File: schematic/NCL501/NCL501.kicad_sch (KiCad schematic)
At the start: 24 parts, among them CN1 SCSI Intern, J1 SCSI extern, J2 Bus_ISA_8bit, U1 74LS175, U10 PAL16L8, U2 74LS125, U3 74LS14, U4 6116, U5 53C80, U6 27C128, U7 74LS688, U8 74LS688, U9 74LS245

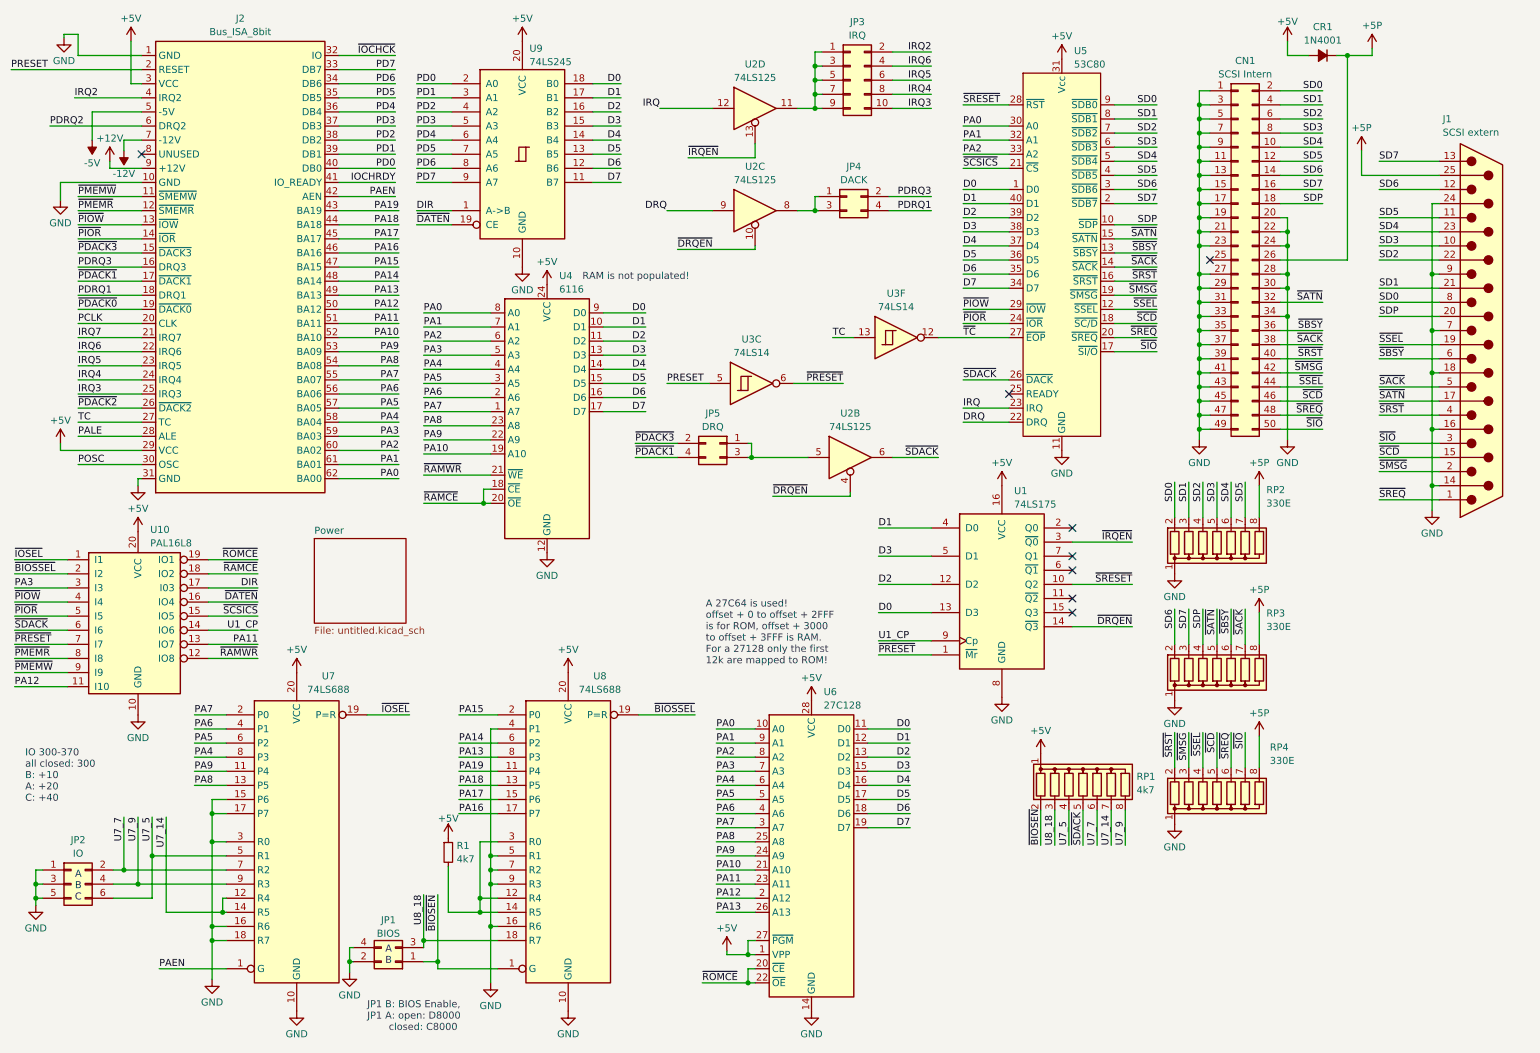
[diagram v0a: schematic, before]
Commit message: first manufactured Version
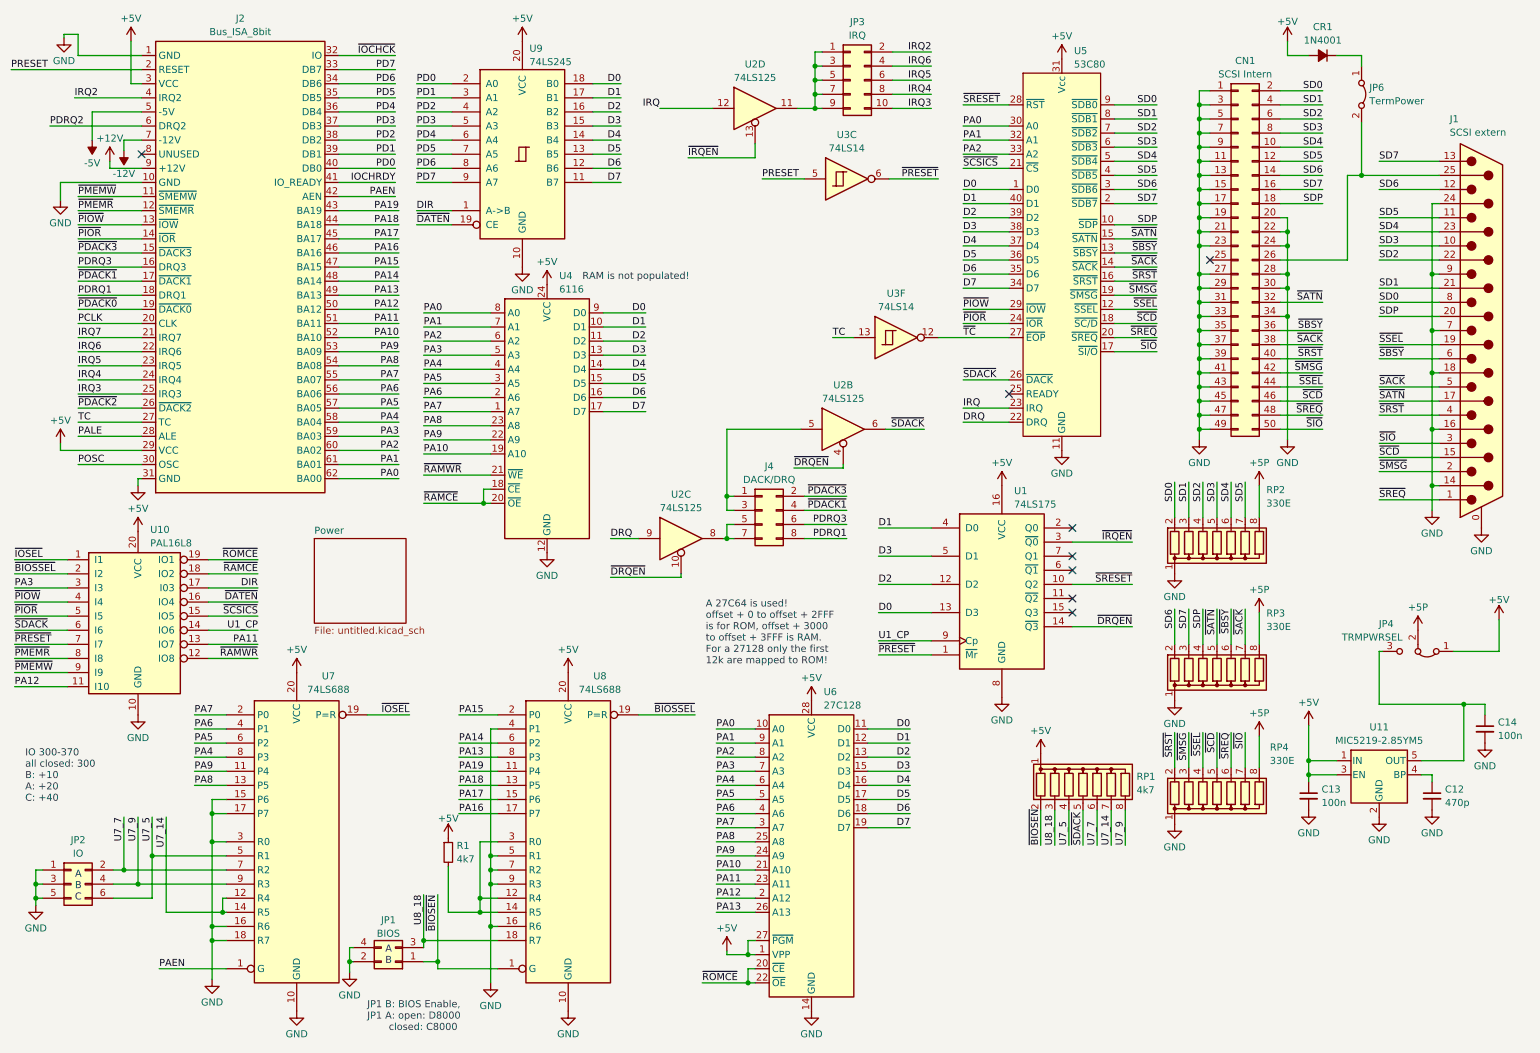
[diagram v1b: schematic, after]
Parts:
- removed J1: SCSI extern, Connector_Dsub:DSUB-25_Female_Horizontal_P2.77x2.54mm_EdgePinOffset9.40mm, symbol Connector:DB25_Plug
- removed JP4: DACK, Connector_PinHeader_2.54mm:PinHeader_2x02_P2.54mm_Vertical, symbol Connector_Generic:Conn_02x02_Odd_Even
- removed JP5: DRQ, Connector_PinHeader_2.54mm:PinHeader_2x02_P2.54mm_Vertical, symbol Connector_Generic:Conn_02x02_Odd_Even
- added C12: 470p, Capacitor_SMD:C_1206_3216Metric_Pad1.33x1.80mm_HandSolder, symbol Device:C_Small
- added C13, C14: 100n, Capacitor_SMD:C_1206_3216Metric_Pad1.33x1.80mm_HandSolder, symbol Device:C_Small
- added J1: SCSI extern, Connector_Dsub:DSUB-25_Female_Horizontal_P2.77x2.84mm_EdgePinOffset7.70mm_Housed_MountingHolesOffset9.12mm, symbol Connector:DB25_Plug_MountingHoles
- added J4: DACK/DRQ, Connector_PinHeader_2.54mm:PinHeader_2x04_P2.54mm_Vertical, symbol Connector_Generic:Conn_02x04_Odd_Even
- added JP4: TRMPWRSEL, Jumper:SolderJumper-3_P1.3mm_Bridged12_RoundedPad1.0x1.5mm, symbol Jumper:Jumper_3_Bridged12
- added JP6: TermPower, Connector_PinHeader_2.54mm:PinHeader_1x02_P2.54mm_Vertical, symbol Jumper:Jumper_2_Bridged
- added U11: MIC5219-2.85YM5, Package_TO_SOT_SMD:SOT-23-5, symbol Regulator_Linear:MIC5219-2.85YM5
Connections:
- net +5P: now also JP4.2 (C); no longer CN1.26 (Pin_26), CR1.1 (K)
- net +5V: now also C13.1, JP4.1 (A), U11.1 (IN), U11.3 (EN)
- net GND: now also C12.2, C13.2, C14.2, J1.0 (PAD), J1.14 (P14), J1.16 (P16), J1.18 (P18), J1.24 (P24), J1.7, J1.9, U11.2 (GND)
- net PDRQ1: now also J4.8 (Pin_8)
- net PDRQ3: now also J4.6 (Pin_6)
- net SD0: now also J1.8
- net SD1: now also J1.21 (P21)
- net SD2: now also J1.22 (P22)
- net SD3: now also J1.10
- net SD4: now also J1.23 (P23)
- net SD5: now also J1.11
- net SD6: now also J1.12
- net SD7: now also J1.13
- net SDP: now also J1.20 (P20)
- net ~{PDACK1}: now also J4.4 (Pin_4)
- net ~{PDACK3}: now also J4.2 (Pin_2)
- net ~{SACK}: now also J1.5
- net ~{SATN}: now also J1.17 (P17)
- net ~{SBSY}: now also J1.6
- net ~{SCD}: now also J1.15 (P15)
- net ~{SIO}: now also J1.3
- net ~{SMSG}: now also J1.2
- net ~{SREQ}: now also J1.1
- net ~{SRST}: now also J1.4
- net ~{SSEL}: now also J1.19 (P19)
- net at U2.5: now also J4.1 (Pin_1), J4.3 (Pin_3)
- net at U2.8: now also J4.5 (Pin_5), J4.7 (Pin_7)
- new net: C14.1, JP4.3 (B), U11.5 (OUT)
- new net: CN1.26 (Pin_26), J1.25 (P25), JP6.2 (B)
- new net: C12.1, U11.4 (BP)
- new net: CR1.1 (K), JP6.1 (A)
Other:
- moved on the sheet: U2B, U2C, U3C

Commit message: Schematic updated
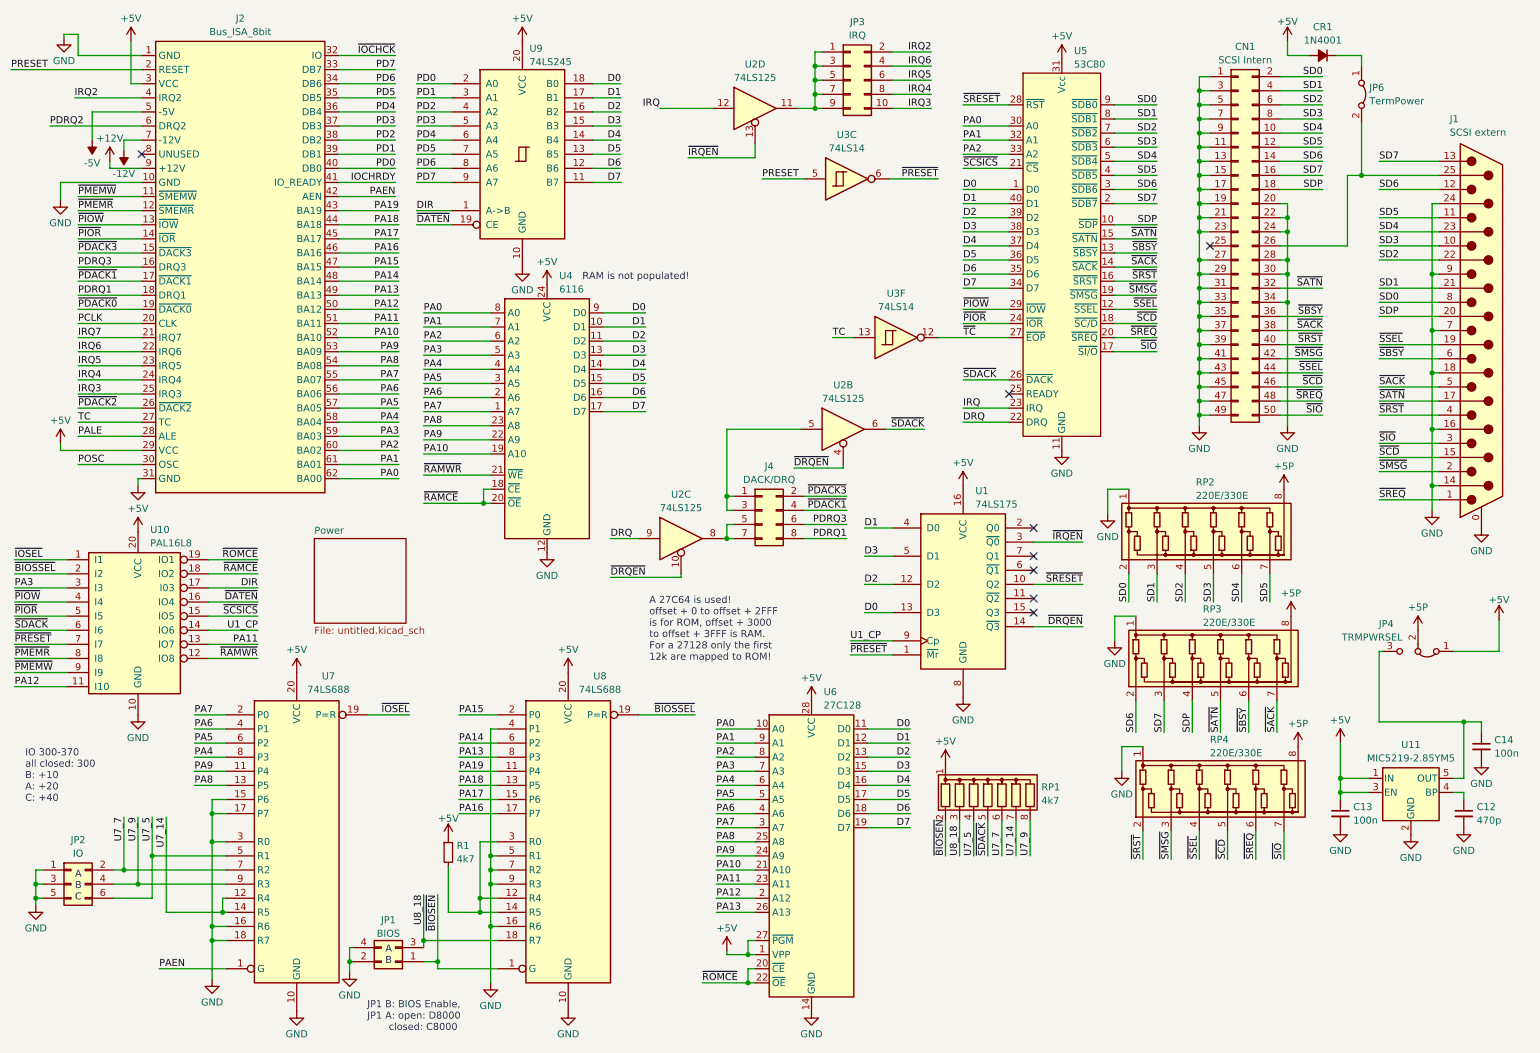
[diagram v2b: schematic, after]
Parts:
- removed RP2, RP3, RP4: 330E, Resistor_THT:R_Array_SIP8, symbol Device:R_Network07
- added RP2, RP3, RP4: 220E/330E, Resistor_THT:R_Array_SIP8, symbol Device:R_Network_Dividers_x06_SIP
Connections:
- net +5P: now also RP2.8 (COM2), RP3.8 (COM2), RP4.8 (COM2)
- net GND: now also RP2.1 (COM1), RP3.1 (COM1), RP4.1 (COM1)
- net SD0: now also RP2.2 (R1)
- net SD1: now also RP2.3 (R2)
- net SD2: now also RP2.4 (R3)
- net SD3: now also RP2.5 (R4)
- net SD4: now also RP2.6 (R5)
- net SD5: now also RP2.7 (R6)
- net SD6: now also RP3.2 (R1)
- net SD7: now also RP3.3 (R2)
- net SDP: now also RP3.4 (R3)
- net ~{SACK}: now also RP3.7 (R6)
- net ~{SATN}: now also RP3.5 (R4)
- net ~{SBSY}: now also RP3.6 (R5)
- net ~{SCD}: now also RP4.5 (R4)
- net ~{SIO}: now also RP4.7 (R6)
- net ~{SMSG}: now also RP4.3 (R2)
- net ~{SREQ}: now also RP4.6 (R5)
- net ~{SRST}: now also RP4.2 (R1)
- net ~{SSEL}: now also RP4.4 (R3)
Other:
- moved on the sheet: C12, C13, C14, CN1, RP1, U1, U11
